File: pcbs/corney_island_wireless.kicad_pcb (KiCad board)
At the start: 2 copper layers, 133.8 x 91.7 mm, 96 parts

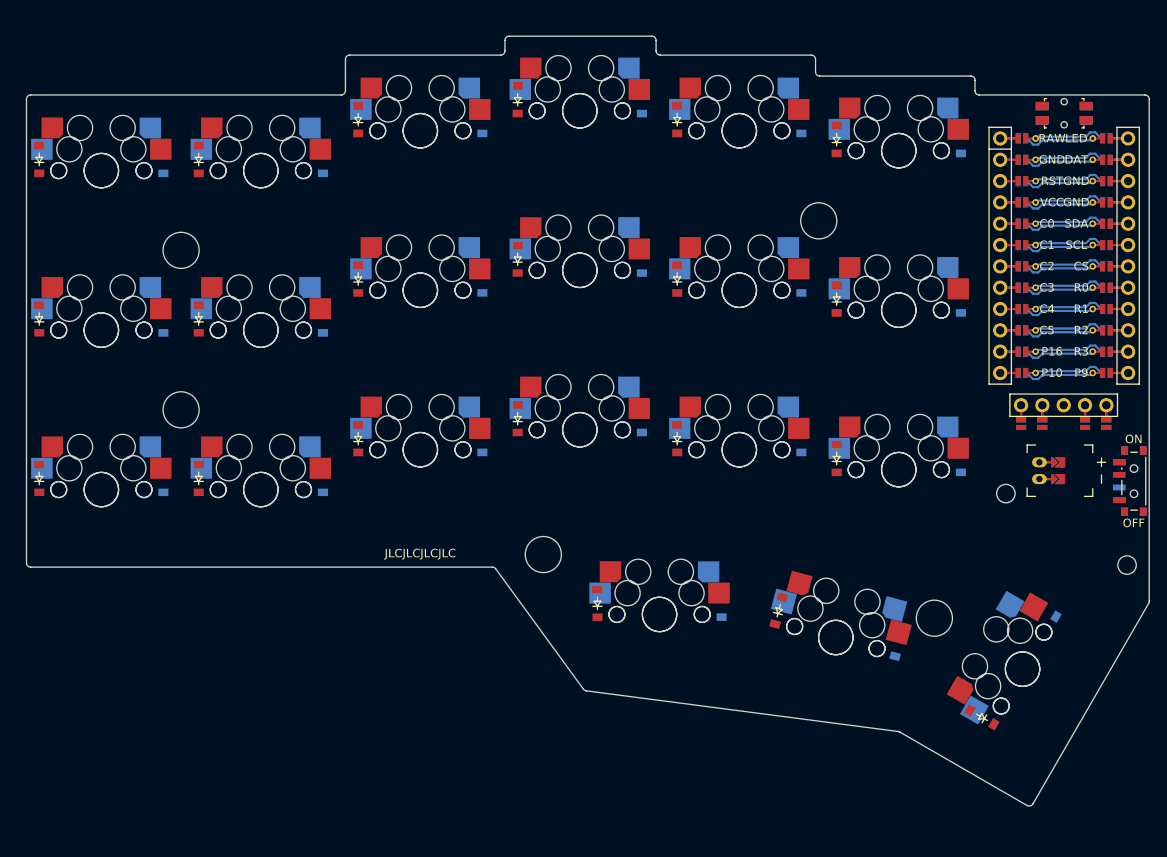
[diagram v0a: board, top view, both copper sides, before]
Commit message: ordered and working nicely.. need some adjustments
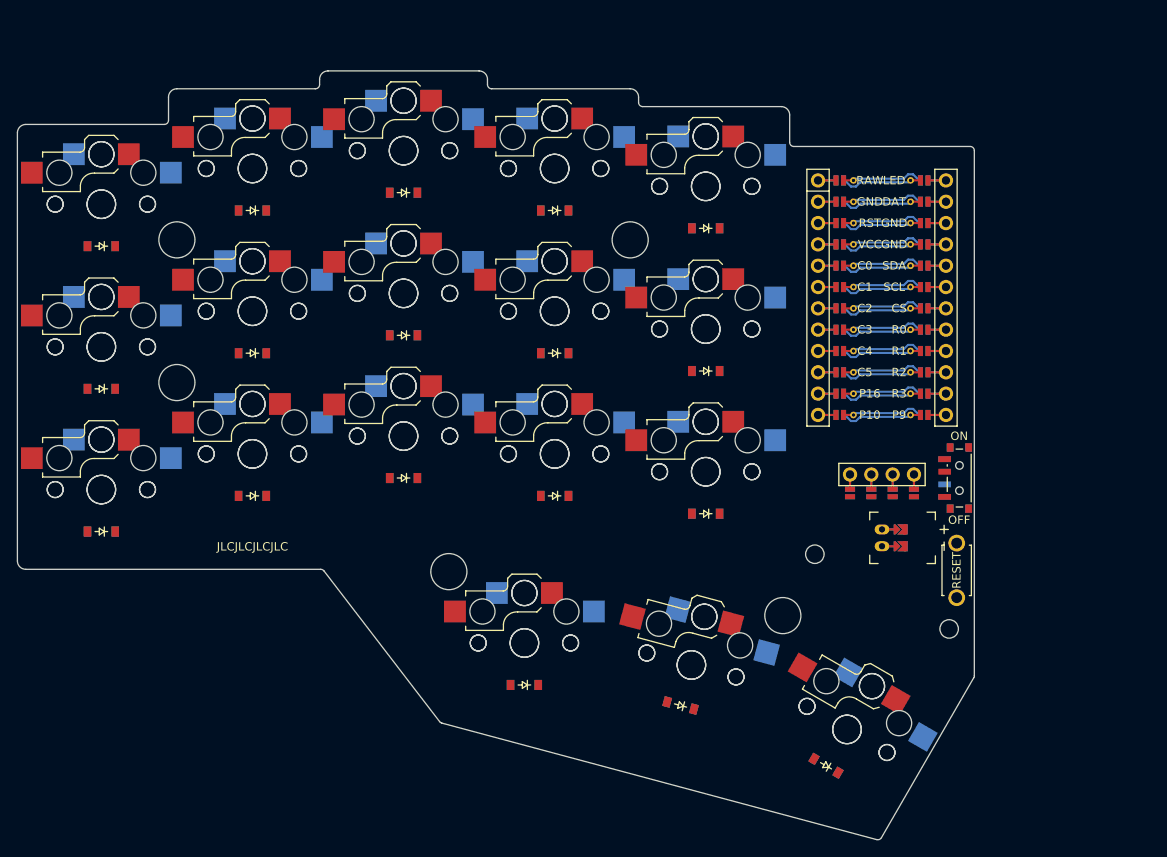
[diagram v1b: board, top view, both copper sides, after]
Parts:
- removed D37, D38, D39, D40, D41, D42: , ceoloide:diode_tht_sod123
- removed RST1: , ceoloide:reset_switch_smd_side
- removed S37, S38, S39, S40, S41, S42: , ceoloide:switch_mx
- added B1: , kbd:ResetSW, F.Cu at (201.9, 109.6)
- D19, D20, D21: moved to F.Cu
- DISP1: footprint ceoloide:display_nice_view -> ceoloide:display_ssd1306
- S1, S10, S11, S12, S13, S14, S15, S16, S17, S18, S2, S22, S23, S24, S25, S26, S27, S28, S29, S3, S30, S31, S32, S33, S34, S35, S36, S4, S5, S6, S7, S8, S9: footprint ceoloide:switch_mx -> ceoloide:switch_choc_v1_v2
- S19, S20, S21: footprint ceoloide:switch_mx -> ceoloide:switch_choc_v1_v2; moved to F.Cu
- moved S21 122.9 mm to (100.0, 66.0), turned to 0 degrees
- moved D21 120.4 mm to (100.0, 71.0), turned to 180 degrees
- moved D20 99.7 mm to (100.0, 88.0), turned to 180 degrees
- moved S20 94.1 mm to (100.0, 83.0), turned to 0 degrees
- moved D36 79.0 mm to (186.3, 132.9), turned to 150 degrees
- moved D18 76.3 mm to (186.3, 132.9), turned to 150 degrees
- moved D19 74.4 mm to (100.0, 105.0), turned to 180 degrees
- moved S36 72.5 mm to (188.8, 128.6), turned to -30 degrees
- moved S18 69.2 mm to (188.8, 128.6), turned to -30 degrees
- moved S19 68.1 mm to (100.0, 100.0)
- moved D17 58.8 mm to (169.0, 125.7), turned to 165 degrees
- moved D16 58.6 mm to (150.4, 123.3), turned to 180 degrees
- moved D35 50.8 mm to (169.0, 125.7), turned to 165 degrees
- moved S16 49.1 mm to (150.4, 118.3)
- moved S17 49.0 mm to (170.3, 120.9), turned to -15 degrees
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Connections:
- D1 pad 2: outer_bottom_B -> pinky_bottom_B
- D10 pad 2: middle_bottom_B -> index_bottom_B
- D11 pad 2: middle_home_B -> index_home_B
- D12 pad 2: middle_top_B -> index_top_B
- D13 pad 2: index_bottom_B -> inner_bottom_B
- D14 pad 2: index_home_B -> inner_home_B
- D15 pad 2: index_top_B -> inner_top_B
- D16 pad 1: R2 -> R3
- D16 pad 2: inner_bottom_B -> near_home_B
- D17 pad 1: R1 -> R3
- D17 pad 2: inner_home_B -> mid_home_B
- D18 pad 1: R0 -> R3
- D18 pad 2: inner_top_B -> far_home_B
- D19 pad 1: R3 -> R2
- D19 pad 2: near_home_B -> pinky_bottom_F
- D2 pad 2: outer_home_B -> pinky_home_B
- D20 pad 1: R3 -> R1
- D20 pad 2: mid_home_B -> pinky_home_F
- D21 pad 1: R3 -> R0
- D21 pad 2: far_home_B -> pinky_top_F
- D22 pad 2: outer_bottom_F -> ring_bottom_F
- D23 pad 2: outer_home_F -> ring_home_F
- D24 pad 2: outer_top_F -> ring_top_F
- D25 pad 2: pinky_bottom_F -> middle_bottom_F
- D26 pad 2: pinky_home_F -> middle_home_F
- D27 pad 2: pinky_top_F -> middle_top_F
- D28 pad 2: ring_bottom_F -> index_bottom_F
- D29 pad 2: ring_home_F -> index_home_F
- D3 pad 2: outer_top_B -> pinky_top_B
- D30 pad 2: ring_top_F -> index_top_F
- D31 pad 2: middle_bottom_F -> inner_bottom_F
- D32 pad 2: middle_home_F -> inner_home_F
- D33 pad 2: middle_top_F -> inner_top_F
- D34 pad 1: R2 -> R3
- D34 pad 2: index_bottom_F -> near_home_F
- D35 pad 1: R1 -> R3
- D35 pad 2: index_home_F -> mid_home_F
- D36 pad 1: R0 -> R3
- D36 pad 2: index_top_F -> far_home_F
- D4 pad 2: pinky_bottom_B -> ring_bottom_B
- D5 pad 2: pinky_home_B -> ring_home_B
- D6 pad 2: pinky_top_B -> ring_top_B
- D7 pad 2: ring_bottom_B -> middle_bottom_B
- D8 pad 2: ring_home_B -> middle_home_B
- D9 pad 2: ring_top_B -> middle_top_B
- DISP1 pad 10: CS -> GND
- DISP1 pad 11: GND -> VCC
- DISP1 pad 16: DISP1_4 -> DISP1_3
- DISP1 pad 17: DISP1_5 -> DISP1_4
- DISP1 pad 20: CS -> GND
- DISP1 pad 21: GND -> VCC
- DISP1 pad 24: DISP1_5 -> DISP1_4
- DISP1 pad 25: DISP1_4 -> DISP1_3
- DISP1 pad 3: VCC -> DISP1_3
- S1 pad 1: C0 -> C1
- S1 pad 2: outer_bottom_B -> pinky_bottom_B
- S10 pad 1: C3 -> C4
- S10 pad 2: middle_bottom_B -> index_bottom_B
- S11 pad 1: C3 -> C4
- S11 pad 2: middle_home_B -> index_home_B
- S12 pad 1: C3 -> C4
- S12 pad 2: middle_top_B -> index_top_B
- S13 pad 1: C4 -> C5
- S13 pad 2: index_bottom_B -> inner_bottom_B
- S14 pad 1: C4 -> C5
- S14 pad 2: index_home_B -> inner_home_B
- S15 pad 1: C4 -> C5
- S15 pad 2: index_top_B -> inner_top_B
- S16 pad 1: C5 -> C3
- S16 pad 2: inner_bottom_B -> near_home_B
- S17 pad 1: C5 -> C4
- S17 pad 2: inner_home_B -> mid_home_B
- S18 pad 2: inner_top_B -> far_home_B
- S19 pad 1: C3 -> C1
- S19 pad 2: near_home_B -> pinky_bottom_F
- S2 pad 1: C0 -> C1
- S2 pad 2: outer_home_B -> pinky_home_B
- S20 pad 1: C4 -> C1
- S20 pad 2: mid_home_B -> pinky_home_F
- S21 pad 1: C5 -> C1
- S21 pad 2: far_home_B -> pinky_top_F
- S22 pad 1: C0 -> C2
- S22 pad 2: outer_bottom_F -> ring_bottom_F
- S23 pad 1: C0 -> C2
- S23 pad 2: outer_home_F -> ring_home_F
- S24 pad 1: C0 -> C2
- S24 pad 2: outer_top_F -> ring_top_F
- S25 pad 1: C1 -> C3
- S25 pad 2: pinky_bottom_F -> middle_bottom_F
- S26 pad 1: C1 -> C3
- S26 pad 2: pinky_home_F -> middle_home_F
- S27 pad 1: C1 -> C3
- S27 pad 2: pinky_top_F -> middle_top_F
- S28 pad 1: C2 -> C4
- S28 pad 2: ring_bottom_F -> index_bottom_F
- S29 pad 1: C2 -> C4
- S29 pad 2: ring_home_F -> index_home_F
- S3 pad 1: C0 -> C1
- S3 pad 2: outer_top_B -> pinky_top_B
- S30 pad 1: C2 -> C4
- S30 pad 2: ring_top_F -> index_top_F
- S31 pad 1: C3 -> C5
- S31 pad 2: middle_bottom_F -> inner_bottom_F
- S32 pad 1: C3 -> C5
- S32 pad 2: middle_home_F -> inner_home_F
- S33 pad 1: C3 -> C5
- S33 pad 2: middle_top_F -> inner_top_F
- S34 pad 1: C4 -> C3
- S34 pad 2: index_bottom_F -> near_home_F
- S35 pad 2: index_home_F -> mid_home_F
- S36 pad 1: C4 -> C5
- S36 pad 2: index_top_F -> far_home_F
- S4 pad 1: C1 -> C2
- S4 pad 2: pinky_bottom_B -> ring_bottom_B
- S5 pad 1: C1 -> C2
- S5 pad 2: pinky_home_B -> ring_home_B
- S6 pad 1: C1 -> C2
- S6 pad 2: pinky_top_B -> ring_top_B
- S7 pad 1: C2 -> C3
- S7 pad 2: ring_bottom_B -> middle_bottom_B
- S8 pad 1: C2 -> C3
- S8 pad 2: ring_home_B -> middle_home_B
- S9 pad 1: C2 -> C3
- S9 pad 2: ring_top_B -> middle_top_B
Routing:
- net (no net): track 333.1 -> 0.00 mm
- net GND: track 3.50 -> 28.9 mm
- net C3: track 0.00 -> 9.64 mm
- net C1: track 0.00 -> 9.64 mm
- net VCC: track 0.00 -> 9.64 mm
- net RAW: track 0.00 -> 9.64 mm
- net RST: track 0.00 -> 9.64 mm
- net P16: track 0.00 -> 9.64 mm
- net P10: track 0.00 -> 9.64 mm
- net C5: track 0.00 -> 9.64 mm
- net C4: track 0.00 -> 9.64 mm
- net C2: track 0.00 -> 9.64 mm
- net C0: track 0.00 -> 9.64 mm
- net R3: track 0.00 -> 9.63 mm
- net R1: track 0.00 -> 9.63 mm
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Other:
- board size 133.8 x 91.7 mm -> 114 x 91.6 mm

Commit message: staggero_change
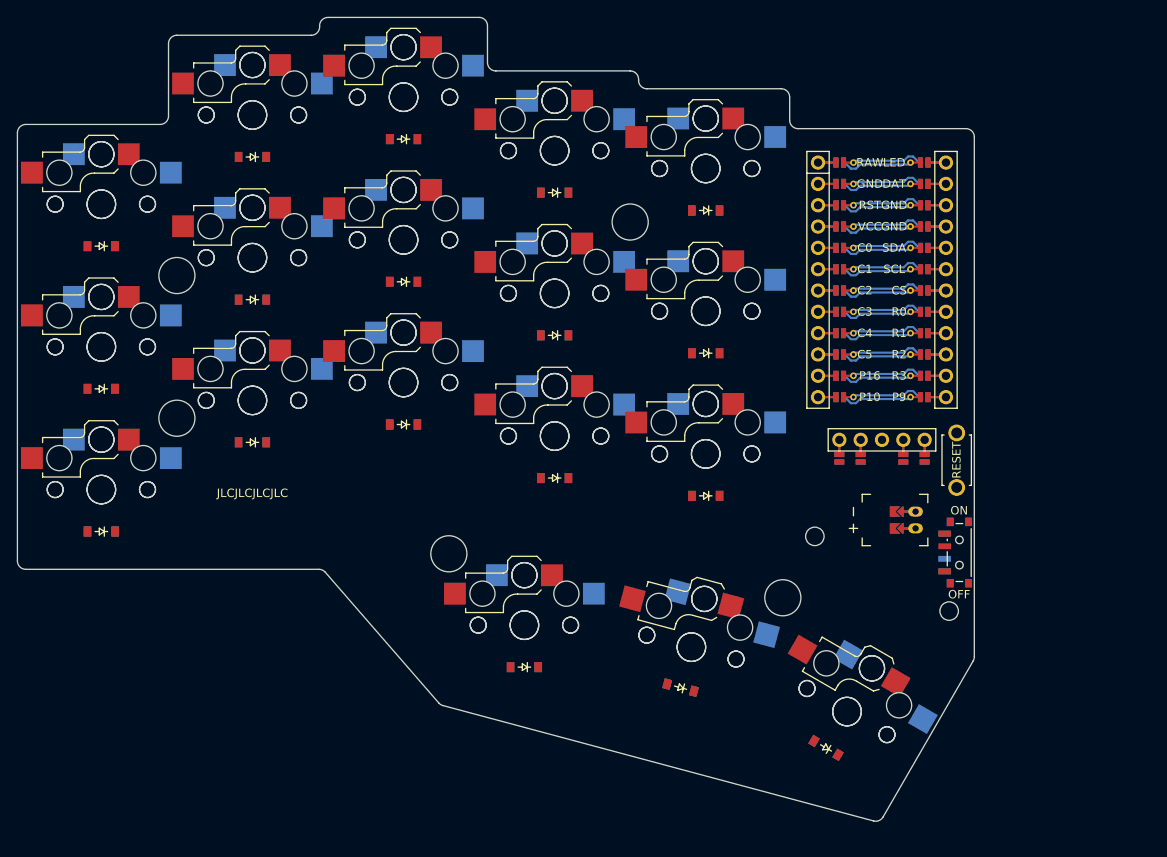
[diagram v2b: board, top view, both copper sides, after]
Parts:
- DISP1: footprint ceoloide:display_ssd1306 -> ceoloide:display_nice_view
- moved B1 13.1 mm to (201.9, 96.5)
- moved PWR1 8.88 mm to (202.2, 107.5)
- moved D22 6.38 mm to (118.0, 94.4)
- moved D23 6.38 mm to (118.0, 77.4)
- moved D24 6.38 mm to (118.0, 60.4)
- moved D25 6.38 mm to (136.0, 92.2)
- moved D26 6.38 mm to (136.0, 75.2)
- moved D27 6.38 mm to (136.0, 58.2)
- moved D4 6.38 mm to (118.0, 94.4)
- moved D5 6.38 mm to (118.0, 77.4)
- moved D6 6.38 mm to (118.0, 60.4)
- moved D7 6.38 mm to (136.0, 92.2)
- moved D8 6.38 mm to (136.0, 75.2)
- moved D9 6.38 mm to (136.0, 58.2)
- moved S22 6.38 mm to (118.0, 89.4)
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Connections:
- DISP1 pad 10: GND -> CS
- DISP1 pad 11: VCC -> GND
- DISP1 pad 12: SCL -> SCK
- DISP1 pad 13: SDA -> MOSI
- DISP1 pad 16: DISP1_3 -> DISP1_4
- DISP1 pad 17: DISP1_4 -> DISP1_5
- DISP1 pad 20: GND -> CS
- DISP1 pad 21: VCC -> GND
- DISP1 pad 22: SCL -> SCK
- DISP1 pad 23: SDA -> MOSI
- DISP1 pad 24: DISP1_4 -> DISP1_5
- DISP1 pad 25: DISP1_3 -> DISP1_4
- DISP1 pad 3: DISP1_3 -> VCC
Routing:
- net DISP1_5: track 0.00 -> 3.50 mm
- net DISP1_3: track 3.50 -> 0.00 mm
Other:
- board size 114 x 91.6 mm -> 114 x 95.8 mm
